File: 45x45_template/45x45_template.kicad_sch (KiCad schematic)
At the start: 10 parts, among them J1 Screw_Terminal_01x02

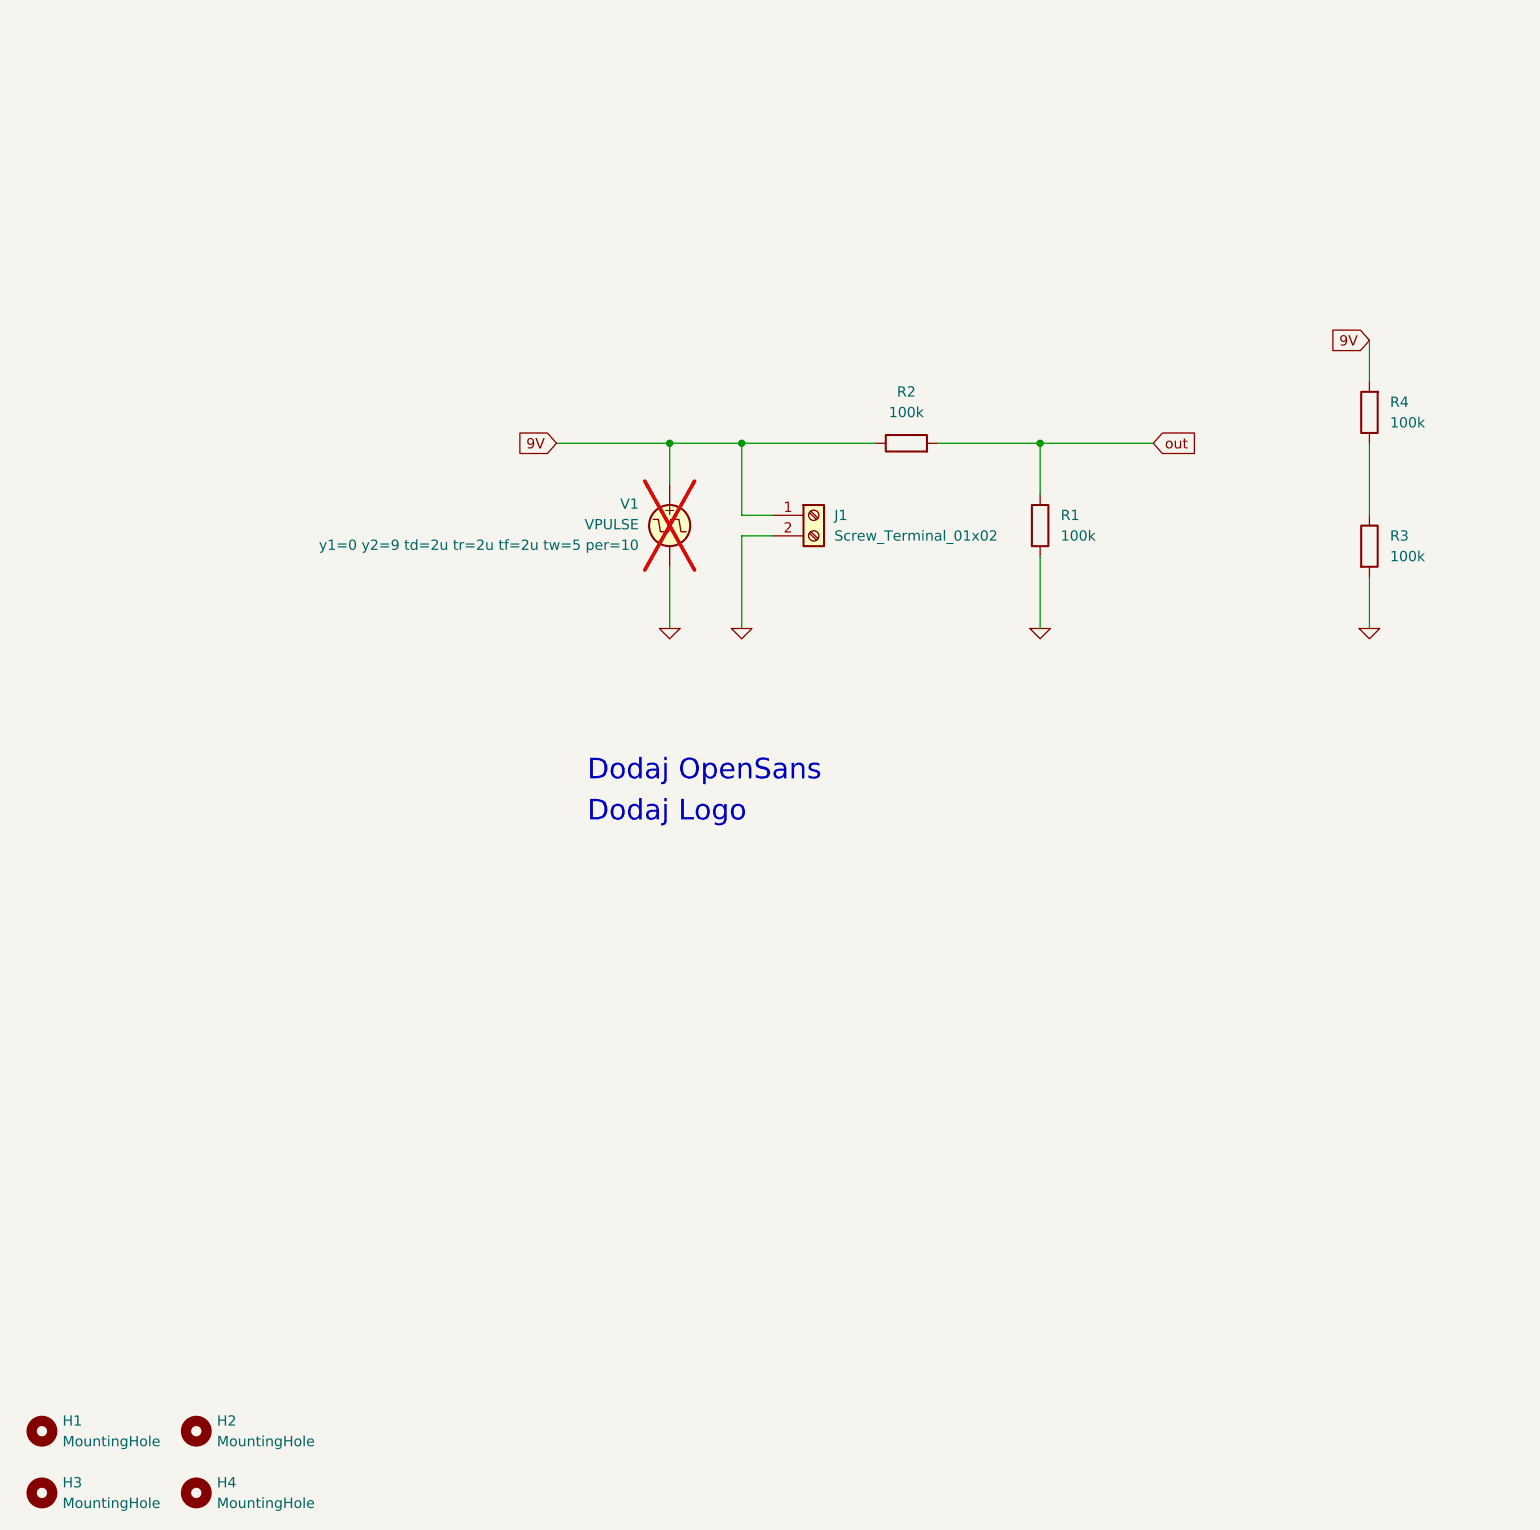
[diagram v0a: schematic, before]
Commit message: Updated template.
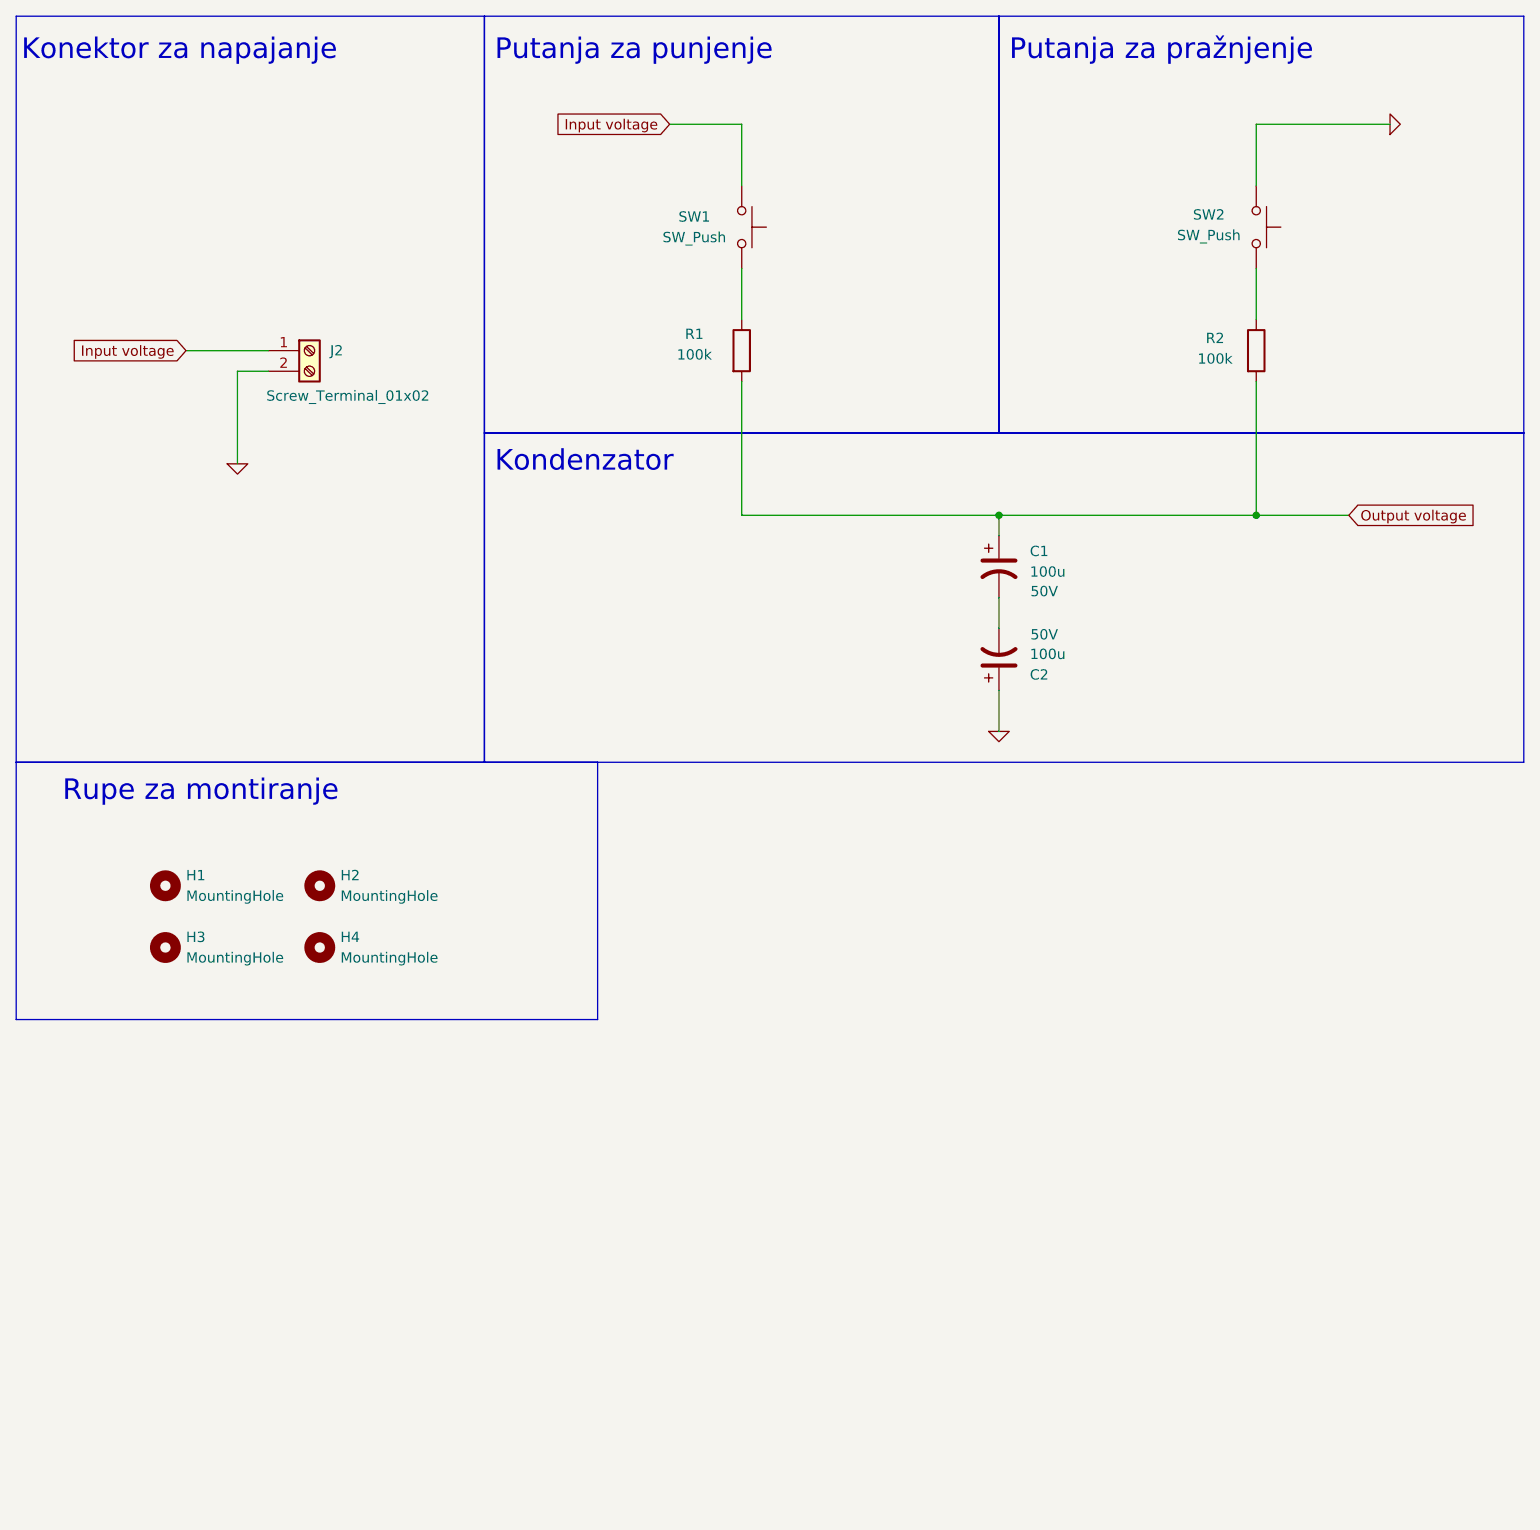
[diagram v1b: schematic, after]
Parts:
- removed J1: Screw_Terminal_01x02, TerminalBlock_Phoenix:TerminalBlock_Phoenix_MKDS-1,5-2-5.08_1x02_P5.08mm_Horizontal, symbol Connector:Screw_Terminal_01x02
- removed R3, R4: 100k, Resistor_THT:R_Axial_DIN0207_L6.3mm_D2.5mm_P15.24mm_Horizontal, symbol Device:R
- removed V1: VPULSE, symbol Simulation_SPICE:VPULSE
- added C1, C2: 100u, Capacitor_THT:CP_Radial_D8.0mm_P3.50mm, symbol Device:C_Polarized_US
- added J2: Screw_Terminal_01x02, TerminalBlock_Phoenix:TerminalBlock_Phoenix_MKDS-1,5-2-5.08_1x02_P5.08mm_Horizontal, symbol Connector:Screw_Terminal_01x02
- added SW1, SW2: SW_Push, Button_Switch_THT:SW_PUSH_6mm_H4.3mm, symbol Switch:SW_Push
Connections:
- net 0: now also C2.1, J2.2 (Pin_2), SW2.1; no longer R1.2
- net 9V: no longer names the net of R2.1
- net 9V: now also SW2.2
- net out: no longer names the net of R1.1
- net out: now also SW1.2; no longer R2.2
- new net: C1.2, C2.2
- new net Input voltage: J2.1 (Pin_1), SW1.1
- new net Output voltage: C1.1, R1.2, R2.2
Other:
- note added: "Kondenzator"
- note added: "Konektor za napajanje"
- note added: "Putanja za pražnjenje"
- note added: "Putanja za punjenje"
- note added: "Rupe za montiranje"
- note removed: "Dodaj Logo"
- note removed: "Dodaj OpenSans"
- title: (none) -> Redna i paralelna otpornost
- moved on the sheet: H1, H2, H3, H4
